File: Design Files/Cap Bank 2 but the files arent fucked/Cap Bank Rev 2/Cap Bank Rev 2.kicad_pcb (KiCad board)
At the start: 2 copper layers, 54 x 85.6 mm, 23 parts, among them J1 Conn_01x02, Q1 2N3904, Q2 2N3904, Q3 2N3904, Q4 2N3904

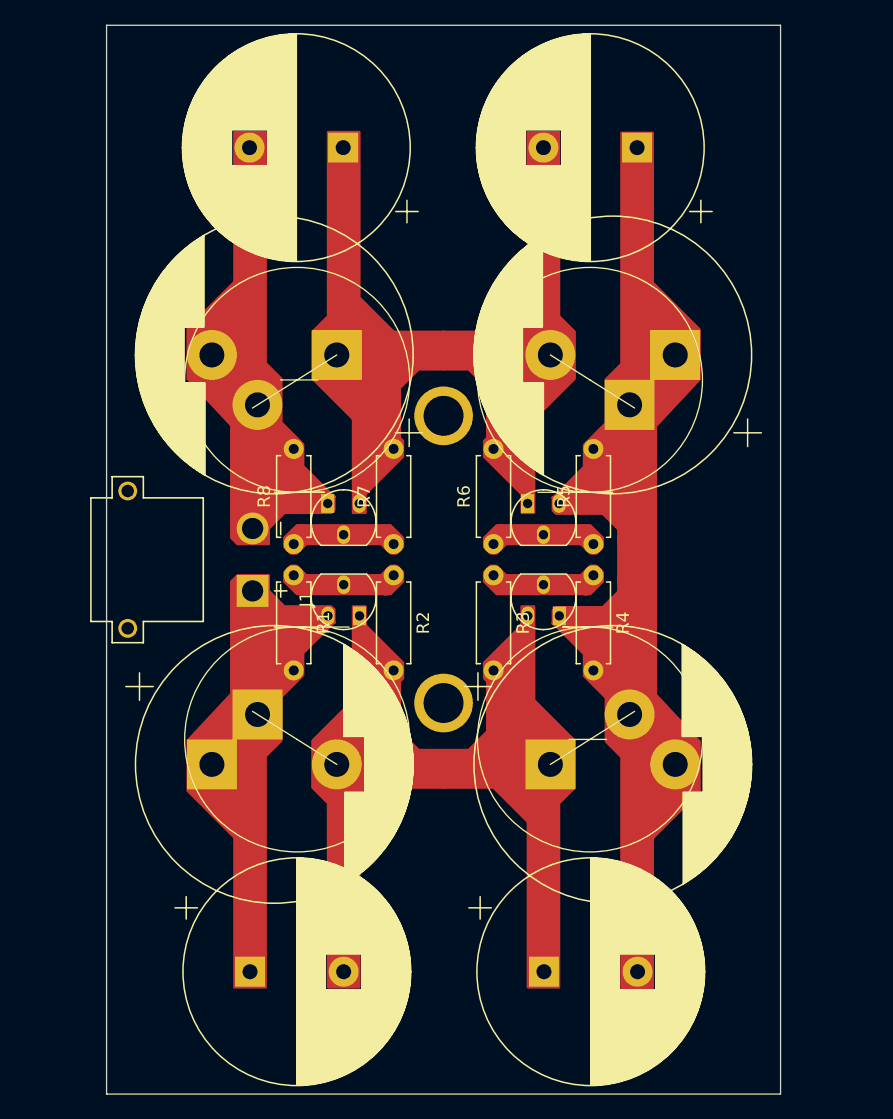
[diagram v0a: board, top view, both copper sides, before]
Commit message: updated again!!!
ship it!
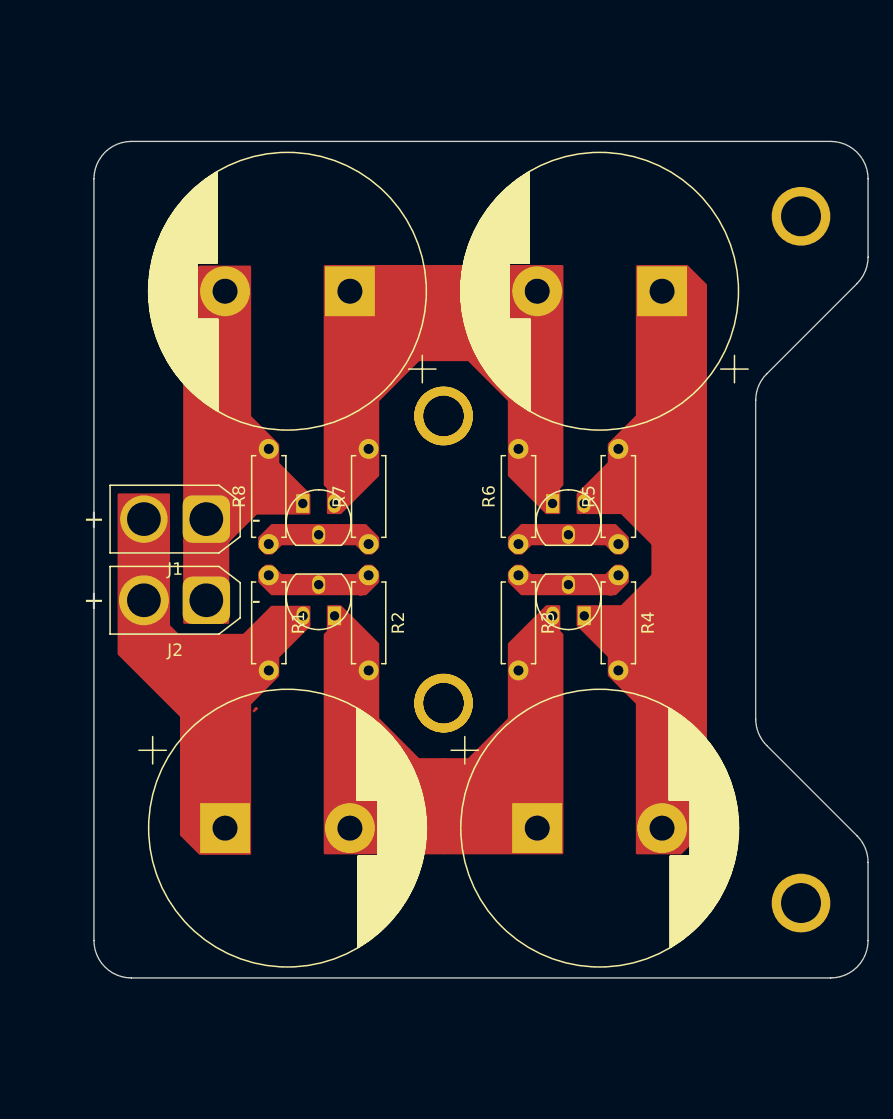
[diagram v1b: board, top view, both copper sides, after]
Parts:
- removed C2, C4, C6, C8: C_Polarized, Library:smallcap
- added ?: , , F.Cu at (150.0, 111.5)
- added ?: , , F.Cu at (178.6, 127.5)
- added ?: , , F.Cu at (150.0, 88.5)
- added ?: , , F.Cu at (178.6, 72.5)
- added J2: Conn_01x02, Connector_AMASS:AMASS_XT30U-F_1x02_P5.0mm_Vertical, F.Cu at (131.0, 103.2)
- C1, C5: footprint Library:bigcap2pos -> Library:bigcap
- C3, C7: footprint Library:bigcap2neg -> Library:bigcap
- J1: footprint Library:xt30 -> Connector_AMASS:AMASS_XT30U-M_1x02_P5.0mm_Vertical
- moved REF** 23.0 mm to (150.0, 111.5)
- moved REF** 23.0 mm to (150.0, 88.5)
- moved J1 7.08 mm to (131.0, 96.8), turned to 180 degrees
- moved C1 5.21 mm to (137.5, 121.5)
- moved C3 5.21 mm to (162.5, 121.5)
- moved C5 5.21 mm to (162.5, 78.5)
- moved C7 5.21 mm to (137.5, 78.5)
- moved Q1 2.00 mm to (140.0, 103.0)
- moved Q2 2.00 mm to (160.0, 103.0)
- moved Q3 2.00 mm to (160.0, 97.0)
- moved Q4 2.00 mm to (140.0, 97.0)
- moved R1 2.00 mm to (136.0, 101.2)
- moved R2 2.00 mm to (144.0, 101.2)
- moved R3 2.00 mm to (156.0, 101.2)
- moved R4 2.00 mm to (164.0, 101.2)
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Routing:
- net /V_IN: track 4.40 -> 0.40 mm
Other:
- board size 54 x 85.6 mm -> 62 x 67 mm

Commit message: new bjt
who dis
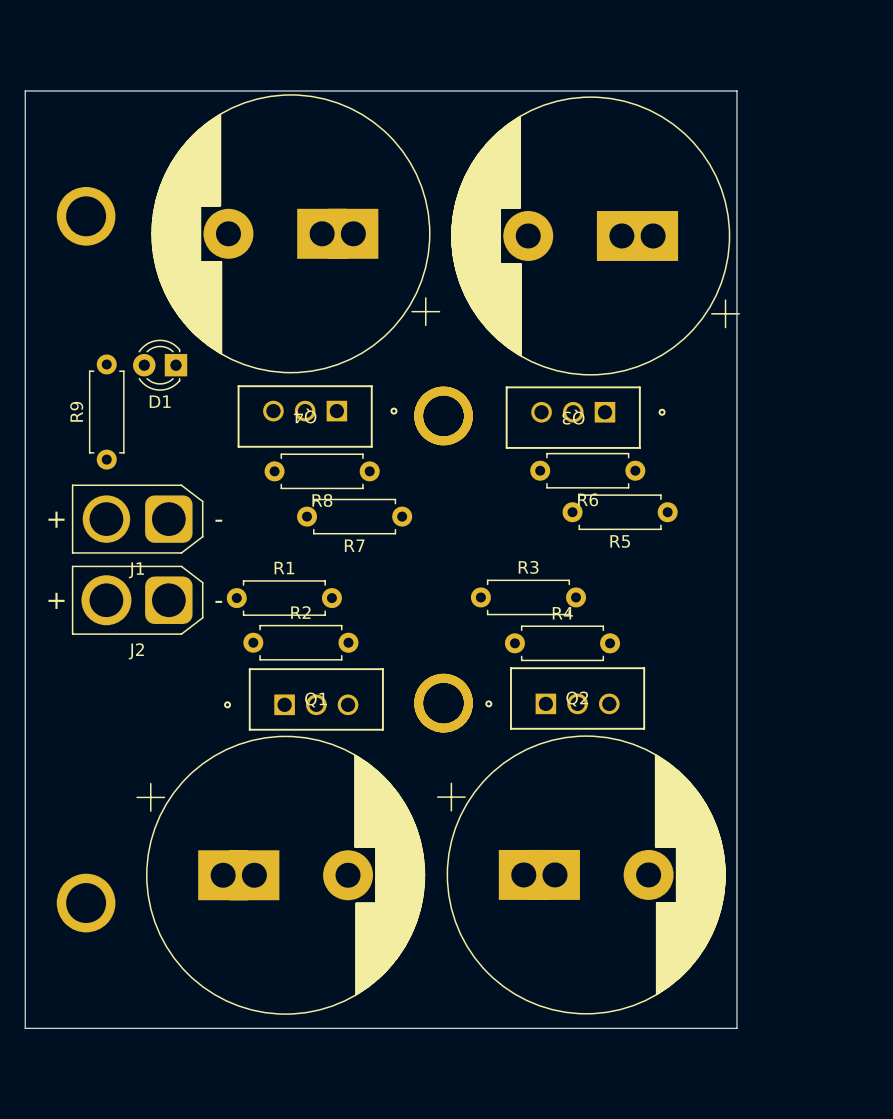
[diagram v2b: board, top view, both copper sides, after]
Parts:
- added D1: LED, LED_THT:LED_D3.0mm_Clear, F.Cu at (128.6, 84.4)
- added R9: 1000, Resistor_THT:R_Axial_DIN0207_L6.3mm_D2.5mm_P7.62mm_Horizontal, F.Cu at (123.0, 92.0)
- Q1, Q2, Q3, Q4: value 2N3904 -> TIP31; footprint Library:2n3904 -> Library:tip31
- moved ? 57.3 mm to (121.4, 127.5)
- moved ? 57.3 mm to (121.4, 72.5)
- moved R6 11.1 mm to (165.4, 92.9), turned to 180 degrees
- moved R2 10.7 mm to (134.8, 106.7), turned to 0 degrees
- moved R8 9.96 mm to (144.1, 92.9), turned to 180 degrees
- moved R4 9.92 mm to (155.7, 106.7), turned to 0 degrees
- moved Q4 8.97 mm to (138.9, 88.1), turned to 180 degrees
- moved Q3 8.82 mm to (160.4, 88.2), turned to 180 degrees
- moved Q1 8.63 mm to (139.8, 111.6), turned to 0 degrees
- moved Q2 8.58 mm to (160.7, 111.5), turned to 0 degrees
- moved R5 4.70 mm to (167.9, 96.2), turned to 180 degrees
- moved C7 4.61 mm to (137.8, 73.9)
- moved C5 4.48 mm to (161.8, 74.1)
- moved C3 3.90 mm to (161.4, 125.2)
- moved C1 3.78 mm to (137.3, 125.3)
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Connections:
- C3 pad 1: Net-(Q1-E) -> Net-(Q2-C)
- C5 pad 1: Net-(Q2-E) -> Net-(Q3-C)
- C7 pad 1: Net-(Q3-E) -> Net-(Q4-C)
- Q1 pad 1: Net-(Q1-E) -> Net-(Q1-B)
- Q1 pad 2: Net-(Q1-B) -> /V_IN
- Q1 pad 3: /V_IN -> Net-(Q1-E)
- Q2 pad 1: Net-(Q2-E) -> Net-(Q2-B)
- Q2 pad 2: Net-(Q2-B) -> Net-(Q2-C)
- Q2 pad 3: Net-(Q1-E) -> Net-(Q2-E)
- Q3 pad 1: Net-(Q3-E) -> Net-(Q3-B)
- Q3 pad 2: Net-(Q3-B) -> Net-(Q3-C)
- Q3 pad 3: Net-(Q2-E) -> Net-(Q3-E)
- Q4 pad 1: /GND -> Net-(Q4-B)
- Q4 pad 2: Net-(Q4-B) -> Net-(Q4-C)
- Q4 pad 3: Net-(Q3-E) -> /GND
- R3 pad 2: Net-(Q1-E) -> Net-(Q2-C)
- R5 pad 2: Net-(Q2-E) -> Net-(Q3-C)
- R7 pad 2: Net-(Q3-E) -> Net-(Q4-C)
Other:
- board size 62 x 67 mm -> 57 x 75.1 mm
